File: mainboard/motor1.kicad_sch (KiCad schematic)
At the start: 12 parts, among them U1 DRV8323RSRGZT

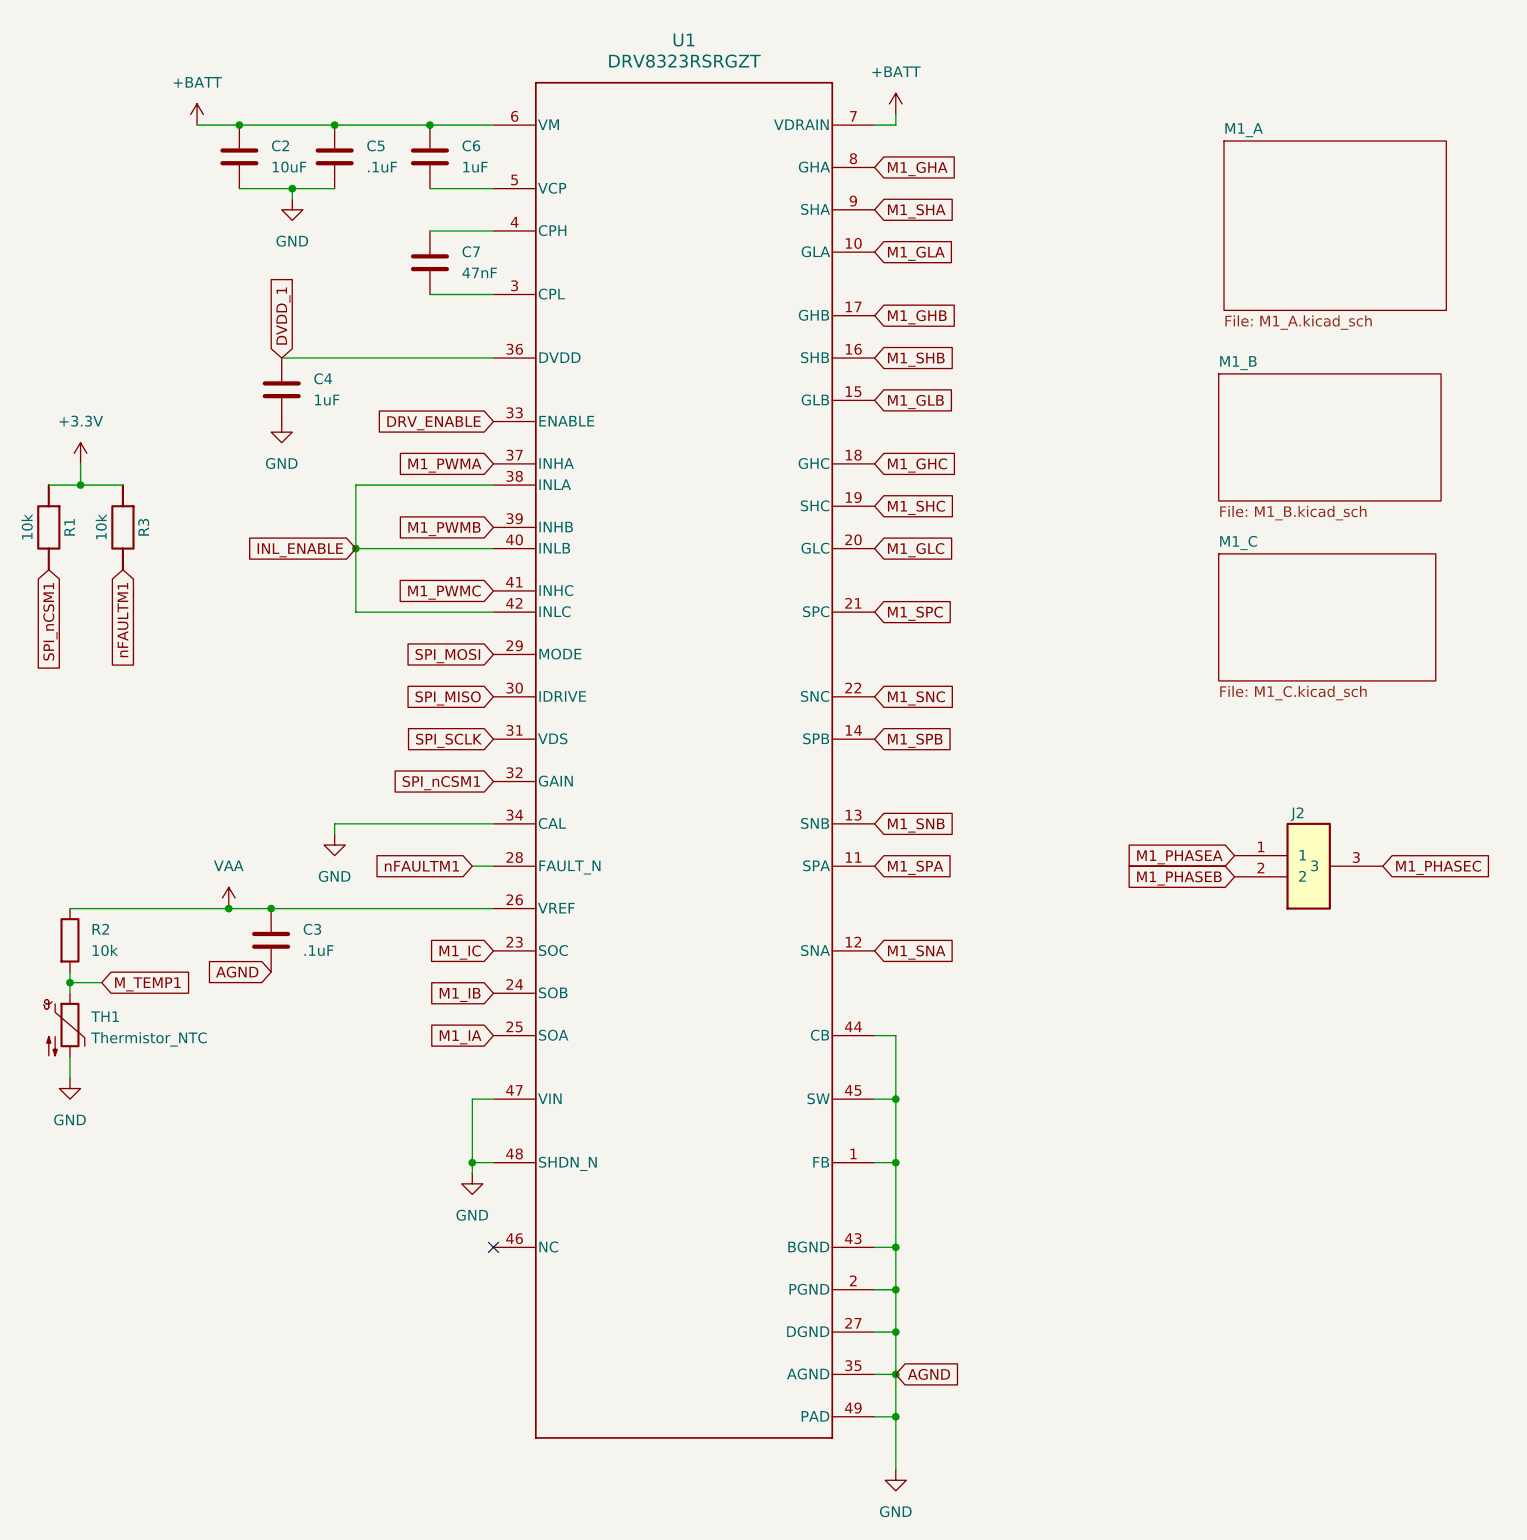
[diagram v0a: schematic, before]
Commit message: Initial layout completed
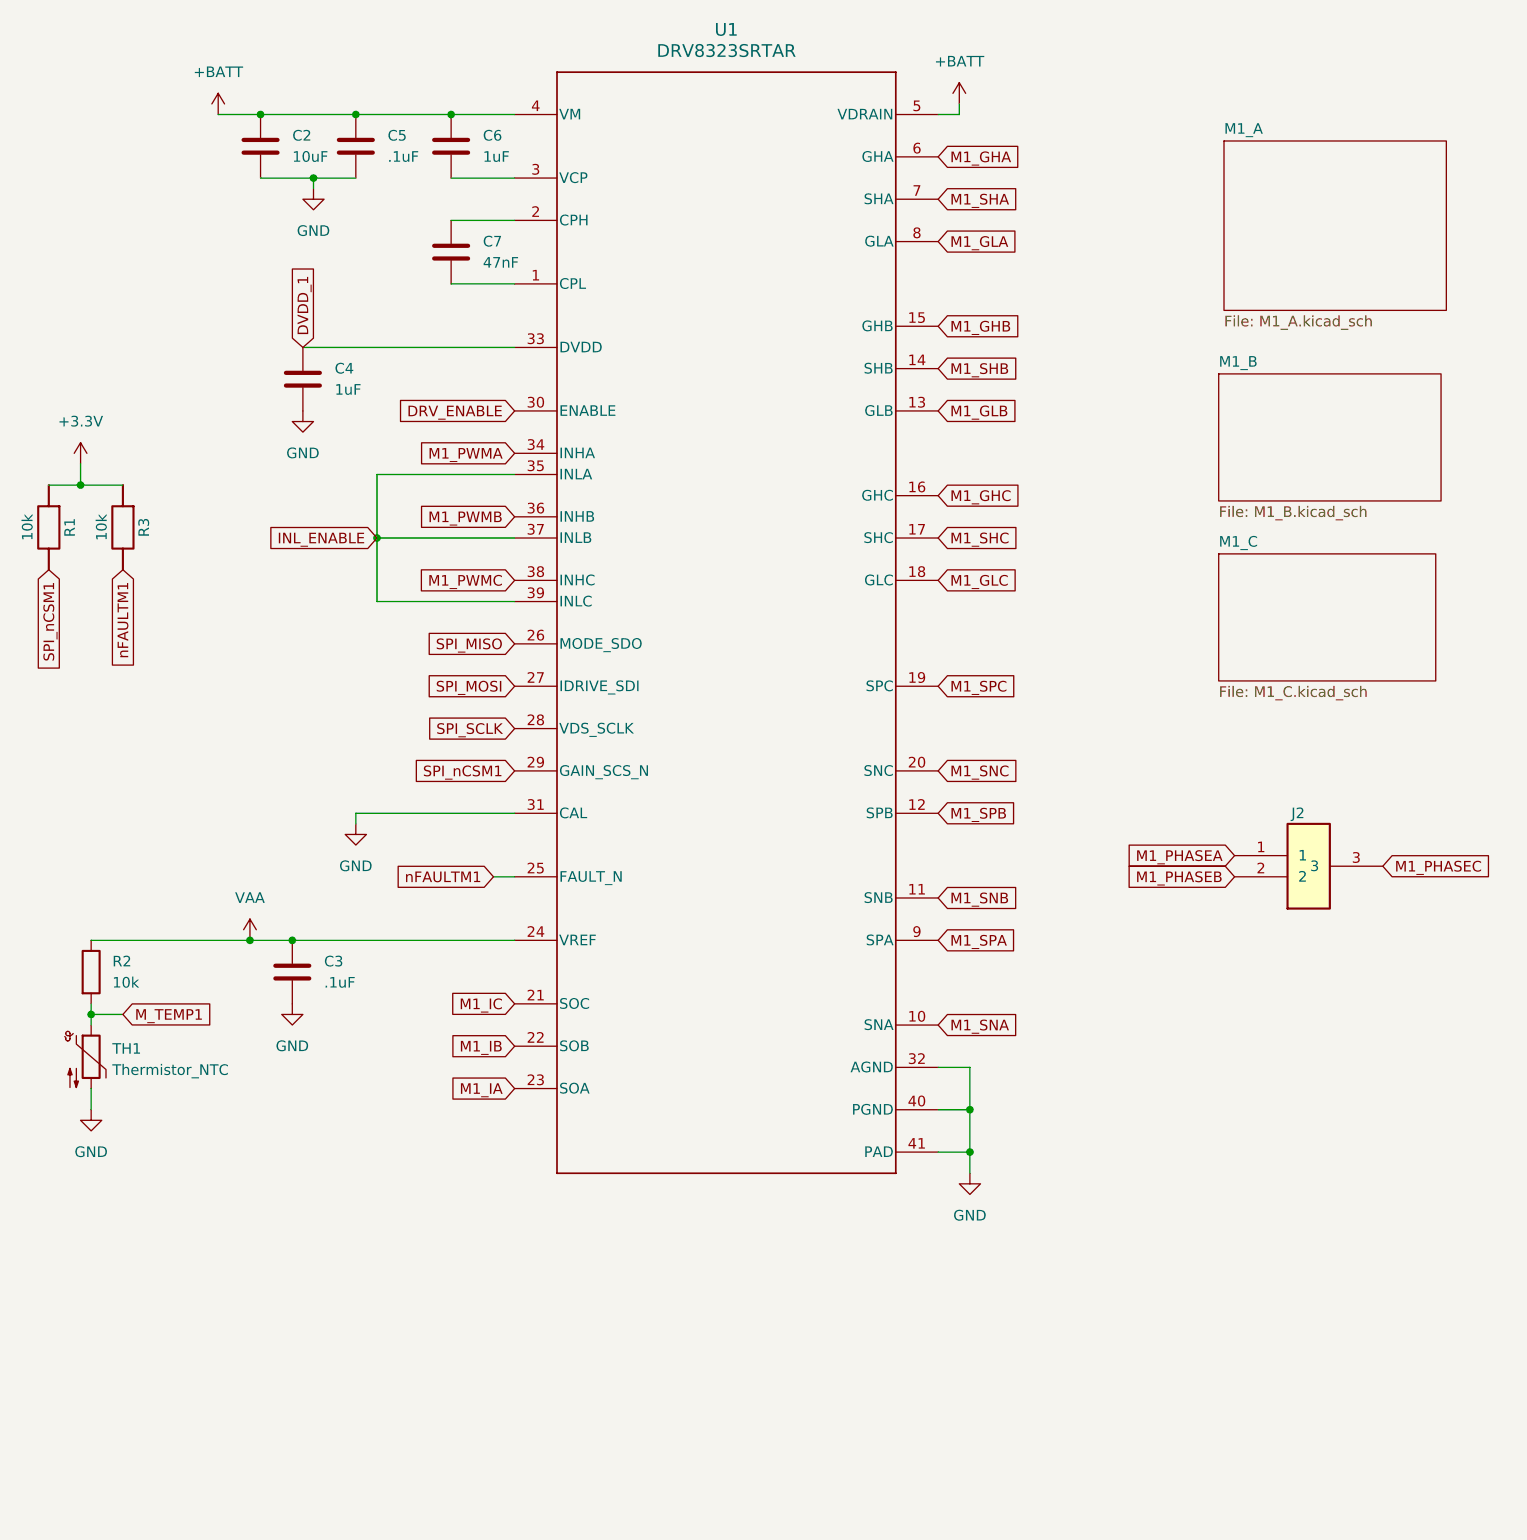
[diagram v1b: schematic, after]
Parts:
- removed U1: DRV8323RSRGZT, DRV8323RSRGZT_new:RGZ0048A, symbol DRV8323RSRGZT_new:DRV8323RSRGZT
- added U1: DRV8323SRTAR, DRV8323SRTAR:RTA0040B_NV, symbol DRV8323SR:DRV8323SRTAR
- C2: footprint Capacitor_SMD:C_1210_3225Metric -> Capacitor_SMD:C_1206_3216Metric
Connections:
- net +BATT: now also U1.4 (VM), U1.5 (VDRAIN)
- net DRV_ENABLE: now also U1.30 (ENABLE)
- net DVDD_1: now also U1.33 (DVDD)
- net GND: now also U1.31 (CAL), U1.32 (AGND), U1.40 (PGND), U1.41 (PAD)
- net INL_ENABLE: now also U1.35 (INLA), U1.37 (INLB), U1.39 (INLC)
- net M1_GHA: now also U1.6 (GHA)
- net M1_GHB: now also U1.15 (GHB)
- net M1_GHC: now also U1.16 (GHC)
- net M1_GLA: now also U1.8 (GLA)
- net M1_GLB: now also U1.13 (GLB)
- net M1_GLC: now also U1.18 (GLC)
- net M1_IA: now also U1.23 (SOA)
- net M1_IB: now also U1.22 (SOB)
- net M1_IC: now also U1.21 (SOC)
- net M1_PWMA: now also U1.34 (INHA)
- net M1_PWMB: now also U1.36 (INHB)
- net M1_PWMC: now also U1.38 (INHC)
- net M1_SHA: now also U1.7 (SHA)
- net M1_SHB: now also U1.14 (SHB)
- net M1_SHC: now also U1.17 (SHC)
- net M1_SNA: now also U1.10 (SNA)
- net M1_SNB: now also U1.11 (SNB)
- net M1_SNC: now also U1.20 (SNC)
- net M1_SPA: now also U1.9 (SPA)
- net M1_SPB: now also U1.12 (SPB)
- net M1_SPC: now also U1.19 (SPC)
- net SPI_MISO: now also U1.26 (MODE_SDO)
- net SPI_MOSI: now also U1.27 (IDRIVE_SDI)
- net SPI_SCLK: now also U1.28 (VDS_SCLK)
- net SPI_nCSM1: now also U1.29 (GAIN_SCS_N)
- net VAA: now also U1.24 (VREF)
- net nFAULTM1: now also U1.25 (FAULT_N)
- net at C6.2: now also U1.3 (VCP)
- net at C7.1: now also U1.2 (CPH)
- net at C7.2: now also U1.1 (CPL)
- no-connect marks 1 -> 0
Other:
- moved on the sheet: C2, C3, C4, C5, C6, C7, R2, TH1
